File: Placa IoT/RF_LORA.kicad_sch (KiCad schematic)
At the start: 1 part, among them U5 T-SX1262

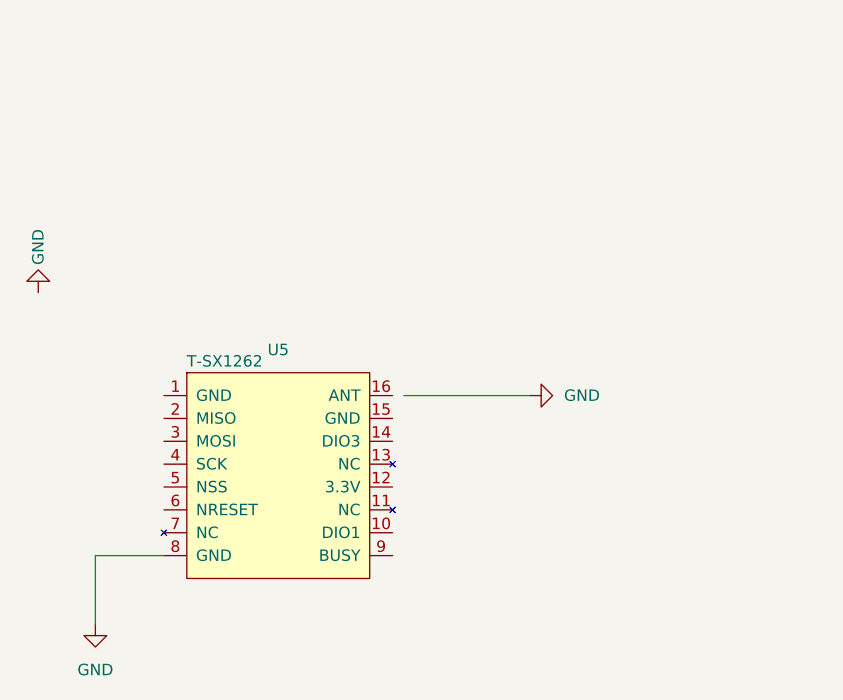
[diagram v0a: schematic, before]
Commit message: RF
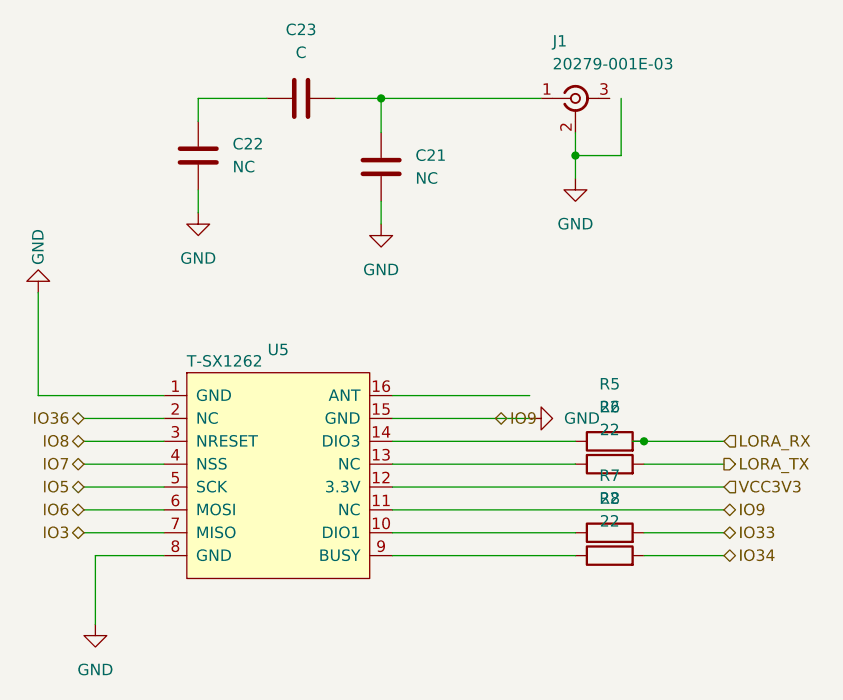
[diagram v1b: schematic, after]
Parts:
- added C21, C22: NC, symbol Device:C
- added C23: C, symbol Device:C
- added J1: 20279-001E-03, antennas:IPEX_MHF_I, symbol antenas:IPEX_MHF_I
- added R5, R6, R7, R8: 22, symbol Device:R
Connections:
- net GND: now also U5.1 (GND), U5.11 (NC), U5.15 (GND), C21.2, C22.2, J1.2 (Ext)
- net at U5.10 (DIO1): now also R7.1
- net VCC3V3: now reaches U5.12 (3.3V)
- net at U5.13 (NC): now also R6.1
- net at U5.14 (DIO3): now also R5.1
- net IO36: now reaches U5.2 (NC)
- net IO8: now reaches U5.3 (NRESET)
- net IO7: now reaches U5.4 (NSS)
- net IO5: now reaches U5.5 (SCK)
- net IO6: now reaches U5.6 (MOSI)
- net IO3: now reaches U5.7 (MISO)
- net at U5.9 (BUSY): now also R8.1
- new net: C22.1, C23.1
- new net: C21.1, C23.2, J1.1 (In)
- new net IO33: R7.2
- new net IO34: R8.2
- new net LORA_RX: R5.2
- new net LORA_TX: R6.2

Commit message: ESQUEMA FINALIZADO
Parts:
- R5, R6, R7, R8: footprint (none) -> Resistor_SMD:R_0402_1005Metric
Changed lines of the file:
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@@
 			)
 		)
-		(property "Footprint" ""
+		(property "Footprint" "Resistor_SMD:R_0402_1005Metric"
 			(at 260.35 93.218 90)
 			(hide yes)
@@
 			)
 		)
-		(property "Footprint" ""
+		(property "Footprint" "Resistor_SMD:R_0402_1005Metric"
 			(at 260.35 100.838 90)
 			(hide yes)
@@
 			)
 		)
-		(property "Footprint" ""
+		(property "Footprint" "Resistor_SMD:R_0402_1005Metric"
 			(at 260.35 103.378 90)
 			(hide yes)
@@
 			)
 		)
-		(property "Footprint" ""
+		(property "Footprint" "Resistor_SMD:R_0402_1005Metric"
 			(at 260.35 90.678 90)
 			(hide yes)

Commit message: ESQUEMA FIN
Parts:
- C21, C22, C23: footprint (none) -> Capacitor_SMD:C_0402_1005Metric
- J1: footprint antennas:IPEX_MHF_I -> antenas:ANTENNA_PIFA_3D_2.4GHZ
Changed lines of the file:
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@@
 			)
 		)
-		(property "Footprint" ""
+		(property "Footprint" "Capacitor_SMD:C_0402_1005Metric"
 			(at 229.87 49.8348 0)
 			(hide yes)
@@
 			)
 		)
-		(property "Footprint" "antennas:IPEX_MHF_I"
+		(property "Footprint" "antenas:ANTENNA_PIFA_3D_2.4GHZ"
 			(at 307.34 20.32 0)
 			(hide yes)
@@
 			)
 		)
-		(property "Footprint" ""
+		(property "Footprint" "Capacitor_SMD:C_0402_1005Metric"
 			(at 235.9152 62.23 0)
 			(hide yes)
@@
 			)
 		)
-		(property "Footprint" ""
+		(property "Footprint" "Capacitor_SMD:C_0402_1005Metric"
 			(at 215.5952 60.96 0)
 			(hide yes)
